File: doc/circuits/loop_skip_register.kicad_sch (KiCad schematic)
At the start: 7 parts, among them U1 74LS193, U10 74LS32, U11 74LS32, U13 74LS193, U6 74LS32, U8 74LS32, U9 74LS32

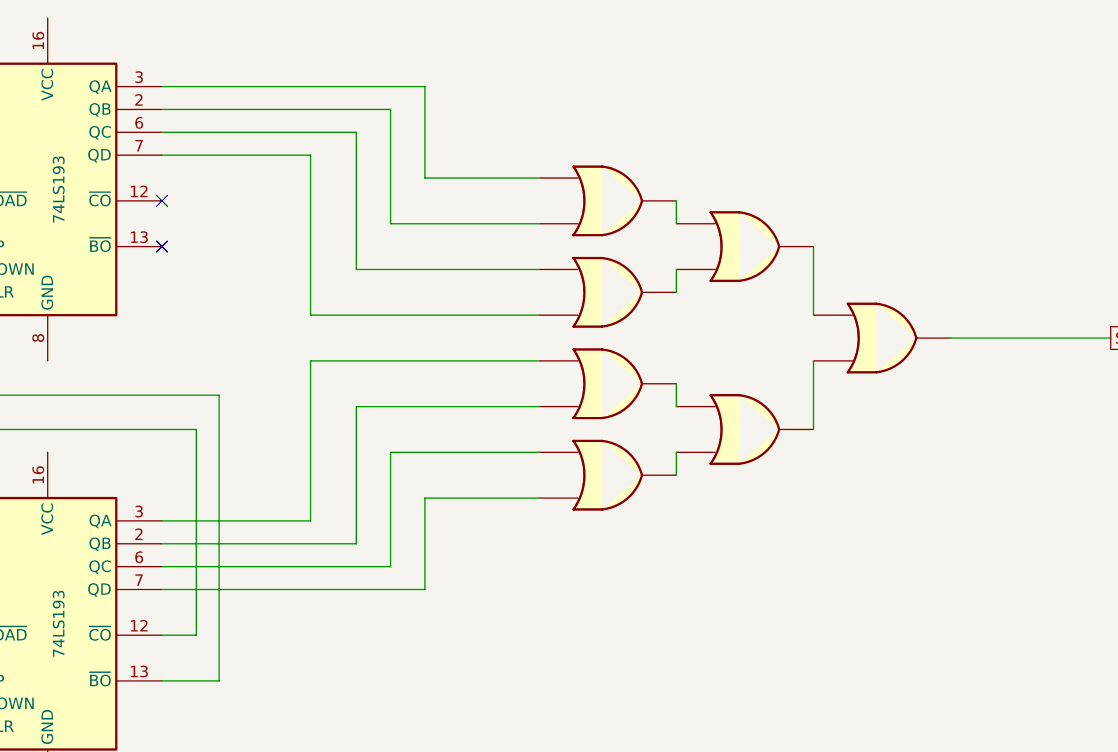
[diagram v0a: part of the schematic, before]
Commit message: more documentation
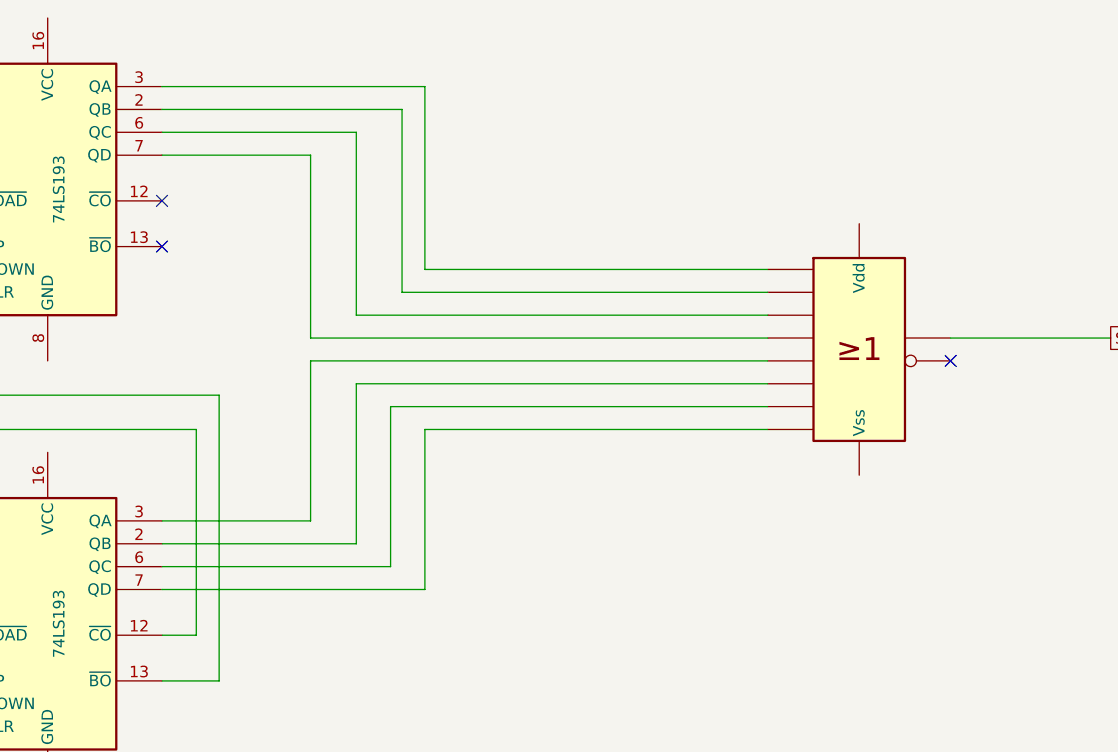
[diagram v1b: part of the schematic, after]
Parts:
- removed U10, U11, U6, U8, U9: 74LS32, symbol 74xx:74LS32
- added U2: 4078, symbol 4xxx_IEEE:4078
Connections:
- net S: now also U2.1
- net at U1.3 (QA): now also U2.2
- net at U1.2 (QB): now also U2.3
- net at U1.6 (QC): now also U2.4
- net at U1.7 (QD): now also U2.5
- net at U13.2 (QB): now also U2.10
- net at U13.3 (QA): now also U2.9
- net at U13.6 (QC): now also U2.11
- net at U13.7 (QD): now also U2.12
- no-connect marks 10 -> 11
